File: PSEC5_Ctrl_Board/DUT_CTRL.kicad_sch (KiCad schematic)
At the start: 2 parts, among them J18 QSH-040-01-X-D-DP-A, J6 QSH-040-01-X-D-DP-A

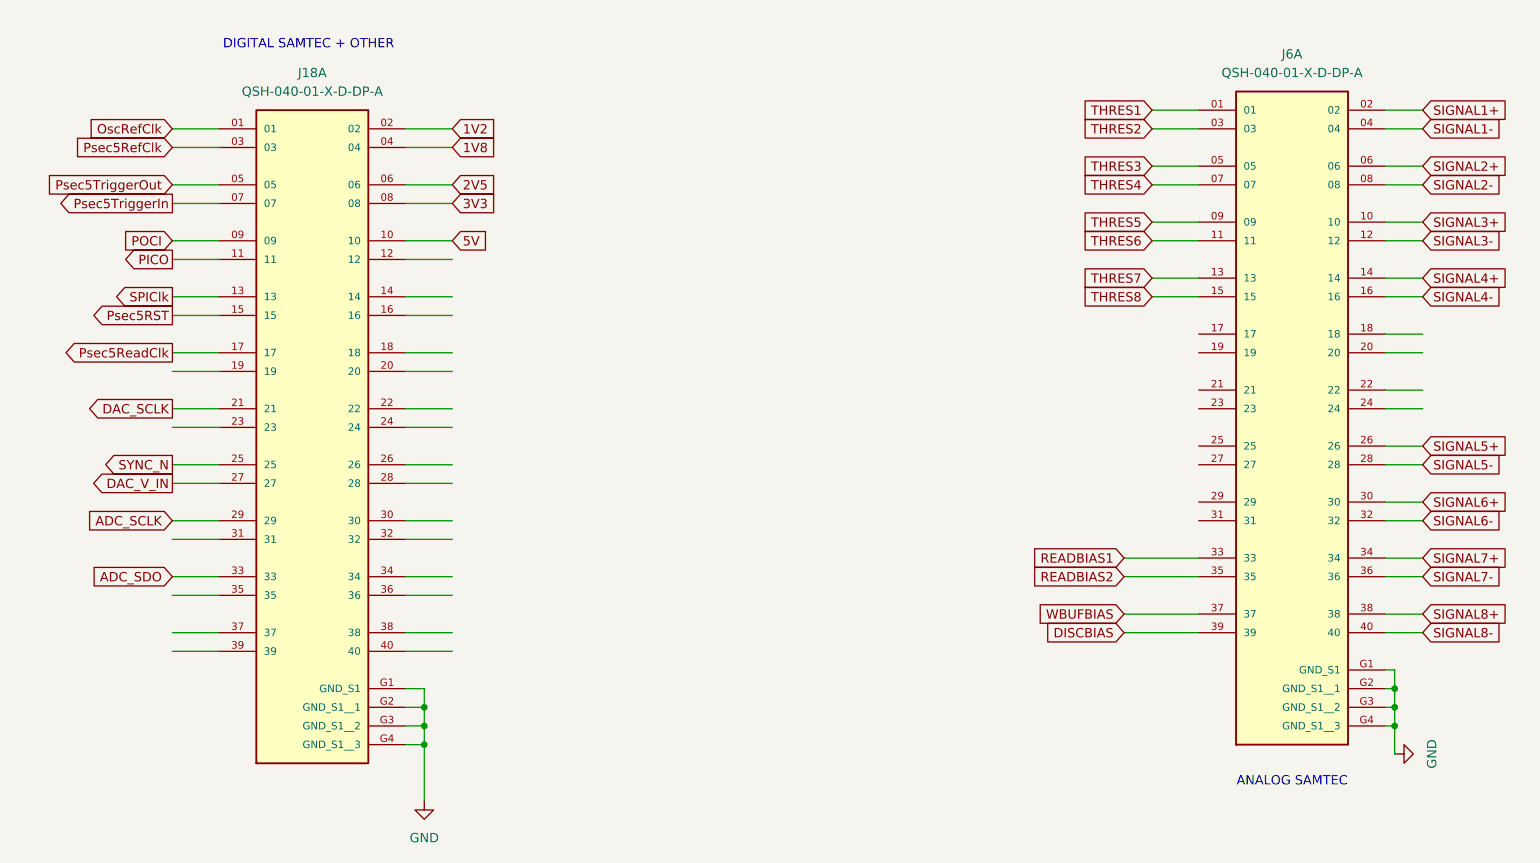
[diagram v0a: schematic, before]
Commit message: minor changes
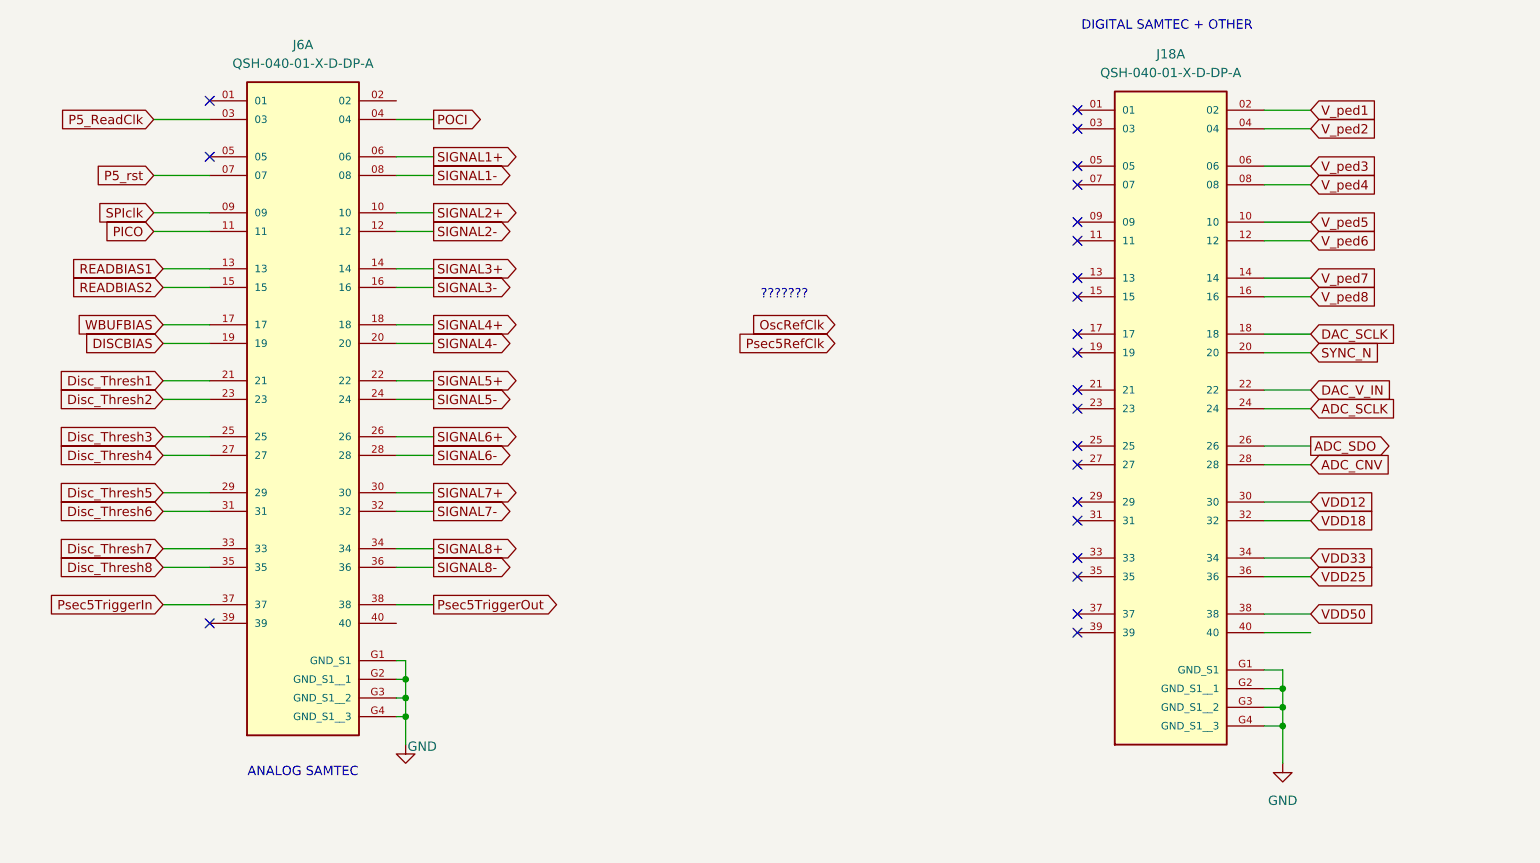
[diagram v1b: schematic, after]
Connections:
- net THRES6 is gone; now on net PICO: J6.11
- net THRES7 is gone; now on net READBIAS1: J6.13
- net THRES8 is gone; now on net READBIAS2: J6.15
- net ADC_SCLK: now also J18.24; no longer J18.29
- net ADC_SDO: now also J18.26; no longer J18.33
- net DAC_SCLK: now also J18.18; no longer J18.21
- net DAC_V_IN: now also J18.22; no longer J18.27
- net DISCBIAS: now also J6.19; no longer J6.39
- net OscRefClk: no longer J18.01
- net PICO: no longer J18.11
- net POCI: now also J6.04; no longer J18.09
- net Psec5RefClk: no longer J18.03
- net Psec5TriggerIn: now also J6.37; no longer J18.07
- net Psec5TriggerOut: now also J6.38; no longer J18.05
- net READBIAS1: no longer J6.33
- net READBIAS2: no longer J6.35
- net SIGNAL1+: now also J6.06; no longer J6.02
- net SIGNAL1-: now also J6.08; no longer J6.04
- net SIGNAL2+: now also J6.10; no longer J6.06
- net SIGNAL2-: now also J6.12; no longer J6.08
- net SIGNAL3+: now also J6.14; no longer J6.10
- net SIGNAL3-: now also J6.16; no longer J6.12
- net SIGNAL4+: now also J6.18; no longer J6.14
- net SIGNAL4-: now also J6.20; no longer J6.16
- net SIGNAL5+: now also J6.22; no longer J6.26
- net SIGNAL5-: now also J6.24; no longer J6.28
- net SIGNAL6+: now also J6.26; no longer J6.30
- net SIGNAL6-: now also J6.28; no longer J6.32
- net SIGNAL7+: now also J6.30; no longer J6.34
- net SIGNAL7-: now also J6.32; no longer J6.36
- net SIGNAL8+: now also J6.34; no longer J6.38
- net SIGNAL8-: now also J6.36; no longer J6.40
- net SYNC_N: now also J18.20; no longer J18.25
- net WBUFBIAS: now also J6.17; no longer J6.37
- net Disc_Thresh1: now reaches J6.21
- net Disc_Thresh2: now reaches J6.23
- net Disc_Thresh3: now reaches J6.25
- net Disc_Thresh4: now reaches J6.27
- net Disc_Thresh5: now reaches J6.29
- net Disc_Thresh6: now reaches J6.31
- net V_ped6: now reaches J18.12
- net V_ped7: now reaches J18.14
- net V_ped8: now reaches J18.16
- net ADC_CNV: now reaches J18.28
- net VDD12: now reaches J18.30
- net VDD18: now reaches J18.32
- net VDD33: now reaches J18.34
- net VDD25: now reaches J18.36
- net VDD50: now reaches J18.38
- net 1V2 renamed V_ped1
- net 1V8 renamed V_ped2
- net 2V5 renamed V_ped3
- net 3V3 renamed V_ped4
- net 5V renamed V_ped5
- net Psec5RST: no longer names the net of J18.15
- net Psec5ReadClk: no longer names the net of J18.17
- net SPIClk: no longer names the net of J18.13
- net THRES1: no longer names the net of J6.01
- net THRES2 renamed P5_ReadClk
- net THRES3: no longer names the net of J6.05
- net THRES4 renamed P5_rst
- net THRES5 renamed SPIclk
- new net Disc_Thresh7: J6.33
- new net Disc_Thresh8: J6.35
- no-connect marks 0 -> 23
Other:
- note added: "???????"
- moved on the sheet: J18A, J6A

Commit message: Schematic is "done" ;( (999+ ERC errors)
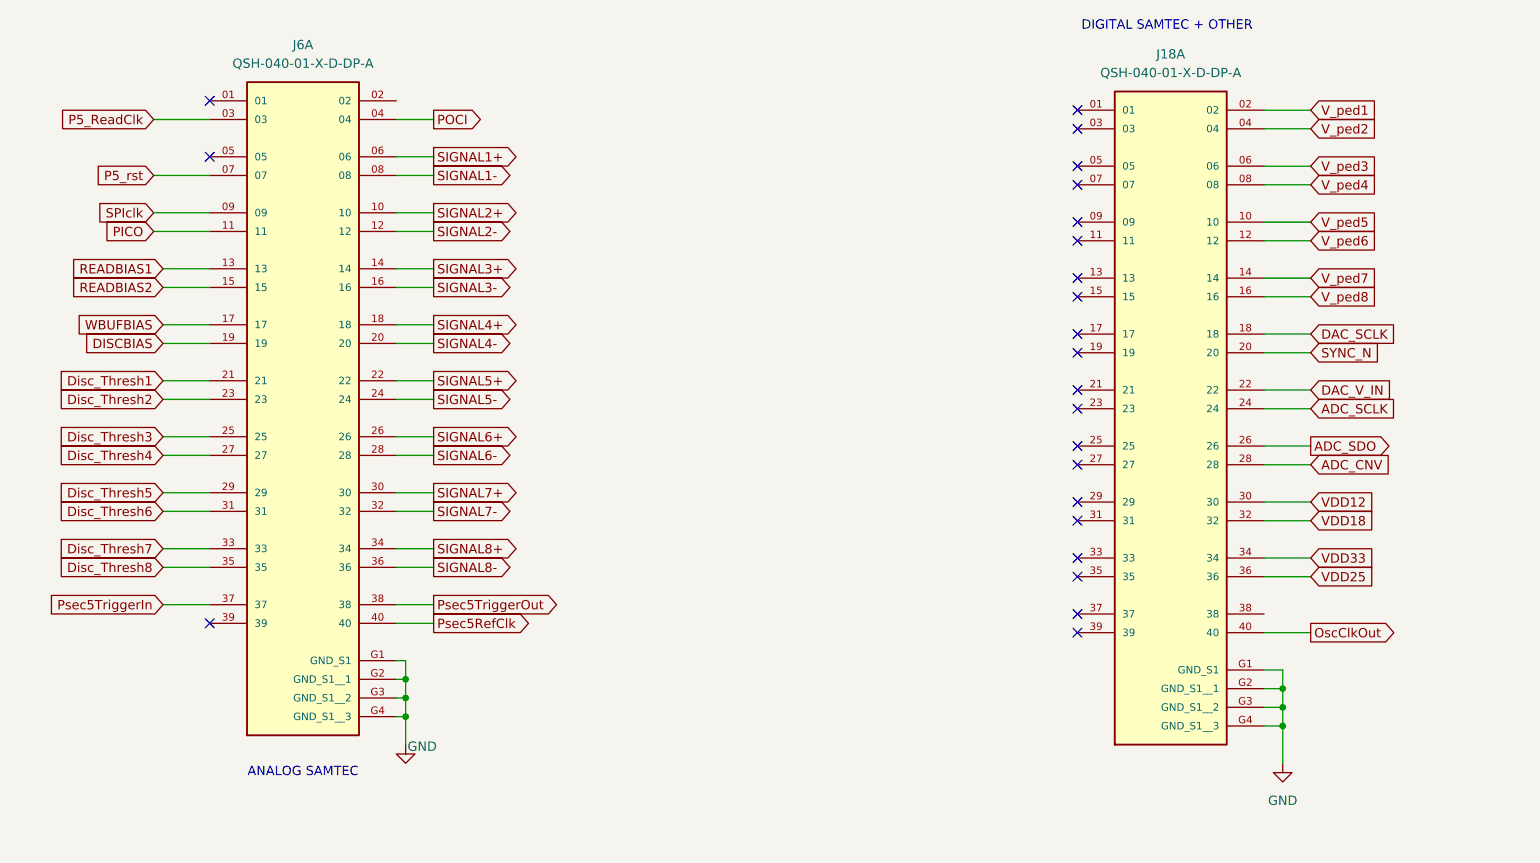
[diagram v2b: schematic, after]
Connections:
- net Psec5RefClk: now also J6.40
- net OscClkOut: now reaches J18.40
- net VDD50: no longer names the net of J18.38
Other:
- note removed: "???????"
